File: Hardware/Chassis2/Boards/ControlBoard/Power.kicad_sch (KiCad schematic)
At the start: 4 parts, among them U7 BTS462TATMA1, U8 BTS462TATMA1

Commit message: update hw revision 7
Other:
- company: (none) -> Corzine Lab, University of California, Santa Cruz
- title: (none) -> Open Inverter Platform - Control Board
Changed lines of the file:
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@@
 	(generator "eeschema")
 	(generator_version "10.0")
-	(paper "A4")
+	(paper "USLetter")
+	(title_block
+		(title "Open Inverter Platform - Control Board")
+		(date "2026-07-07")
+		(rev "G")
+		(company "Corzine Lab, University of California, Santa Cruz")
+		(comment 1 "Prepared by Thomas Liao")
+	)
 	(text "3.3V POWER, 3W MAX"
 		(exclude_from_sim no)

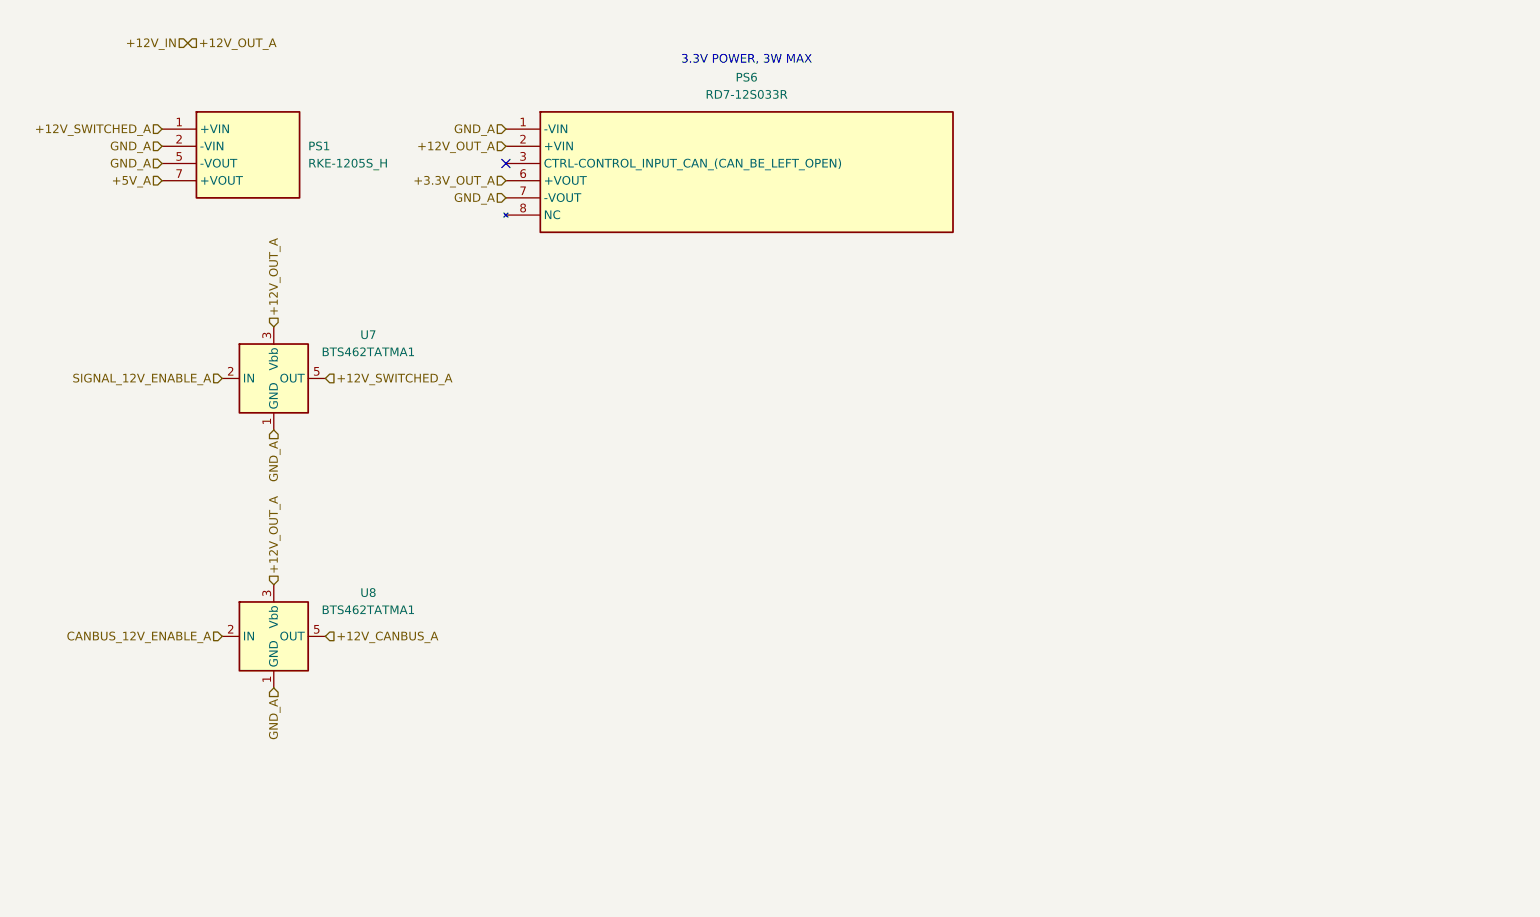
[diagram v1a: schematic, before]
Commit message: eod 2026-07-08
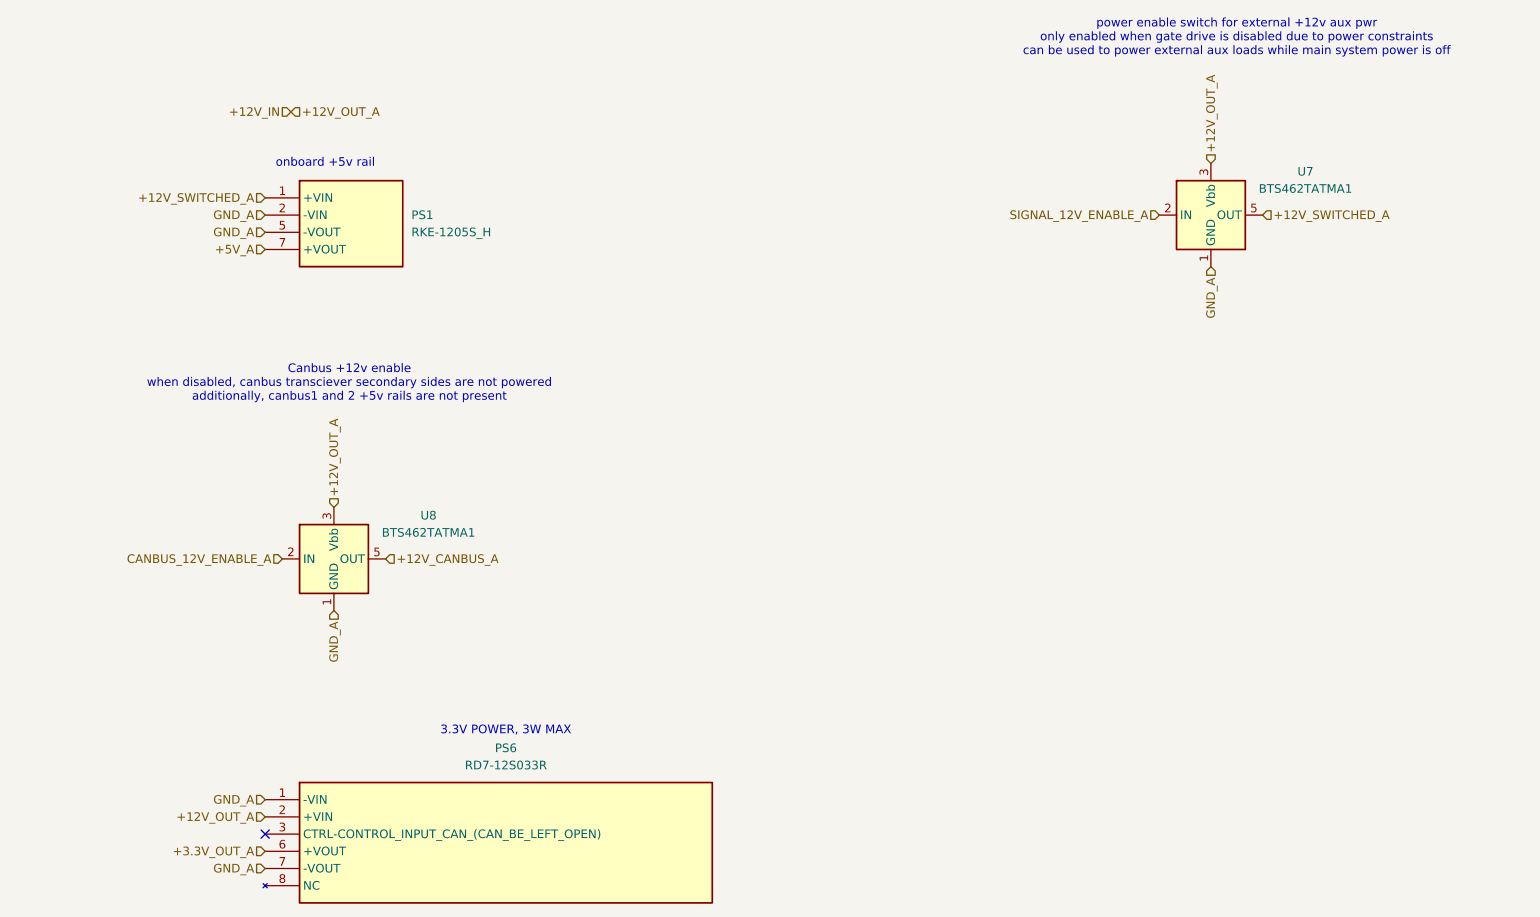
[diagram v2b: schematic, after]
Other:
- note added: "Canbus +12v enable when disabled, canbus transciever secondary sides are not powered additionally, canbus1 and 2 +5v rails are not present"
- note added: "onboard +5v rail"
- note added: "power enable switch for external +12v aux pwr only enabled when gate drive is disabled due to power constraints can be used to power external aux loads while main system power is off"
- moved on the sheet: PS1, PS6, U7, U8
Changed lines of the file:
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@@
 	(text "3.3V POWER, 3W MAX"
 		(exclude_from_sim no)
-		(at 116.84 20.32 0)
+		(at 81.28 119.38 0)
+		(effects
+			(font
+				(size 1.27 1.27)
+			)
+		)
+	)
+	(text "power enable switch for external +12v aux pwr\nonly enabled when gate drive is disabled due to power constraints\ncan be used to power external aux loads while main system power is off"
+		(exclude_from_sim no)
+		(at 189.23 17.018 0)
+		(effects
+			(font
+				(size 1.27 1.27)
+			)
+		)
+	)
+	(text "onboard +5v rail"
+		(exclude_from_sim no)
+		(at 54.61 35.56 0)
+		(effects
+			(font
+				(size 1.27 1.27)
+			)
+		)
+	)
+	(text "Canbus +12v enable\nwhen disabled, canbus transciever secondary sides are not powered\nadditionally, canbus1 and 2 +5v rails are not present"
+		(exclude_from_sim no)
+		(at 58.166 68.072 0)
 		(effects
 			(font
@@
 	)
 	(no_connect
-		(at 81.28 35.56)
+		(at 45.72 134.62)
 	)
 	(hierarchical_label "+12V_OUT_A"
 		(shape input)
-		(at 34.29 17.78 0)
+		(at 49.53 27.94 0)
 		(effects
 			(font
@@
 	(hierarchical_label "CANBUS_12V_ENABLE_A"
 		(shape input)
-		(at 39.37 105.41 180)
+		(at 48.26 93.98 180)
 		(effects
 			(font
@@
 	(hierarchical_label "+12V_SWITCHED_A"
 		(shape input)
-		(at 30.48 30.48 180)
+		(at 45.72 40.64 180)
 		(effects
 			(font
@@
 	(hierarchical_label "+5V_A"
 		(shape input)
-		(at 30.48 38.1 180)
+		(at 45.72 48.26 180)
 		(effects
 			(font
@@
 	(hierarchical_label "GND_A"
 		(shape input)
-		(at 46.99 113.03 270)
+		(at 55.88 101.6 270)
 		(effects
 			(font
@@
 	(hierarchical_label "+12V_OUT_A"
 		(shape input)
-		(at 46.99 59.69 90)
+		(at 185.42 35.56 90)
 		(effects
 			(font
@@
 	(hierarchical_label "GND_A"
 		(shape input)
-		(at 81.28 40.64 180)
+		(at 45.72 139.7 180)
 		(effects
 			(font
@@
 	(hierarchical_label "+12V_CANBUS_A"
 		(shape input)
-		(at 54.61 105.41 0)
+		(at 63.5 93.98 0)
 		(effects
 			(font
@@
 	(hierarchical_label "GND_A"
 		(shape input)
-		(at 30.48 33.02 180)
+		(at 45.72 43.18 180)
 		(effects
 			(font
@@
 	(hierarchical_label "GND_A"
 		(shape input)
-		(at 30.48 35.56 180)
+		(at 45.72 45.72 180)
 		(effects
 			(font
@@
 	(hierarchical_label "+12V_OUT_A"
 		(shape input)
-		(at 46.99 97.79 90)
+		(at 55.88 86.36 90)
 		(effects
 			(font
@@
 	(hierarchical_label "+3.3V_OUT_A"
 		(shape input)
-		(at 81.28 38.1 180)
+		(at 45.72 137.16 180)
 		(effects
 			(font
@@
 	(hierarchical_label "GND_A"
 		(shape input)
-		(at 46.99 74.93 270)
+		(at 185.42 50.8 270)
 		(effects
 			(font
@@
 	(hierarchical_label "+12V_SWITCHED_A"
 		(shape input)
-		(at 54.61 67.31 0)
+		(at 193.04 43.18 0)
 		(effects
 			(font
@@
 	(hierarchical_label "GND_A"
 		(shape input)
-		(at 81.28 30.48 180)
+		(at 45.72 129.54 180)
 		(effects
 			(font
@@
 	(hierarchical_label "+12V_IN"
 		(shape input)
-		(at 34.29 17.78 180)
+		(at 49.53 27.94 180)
 		(effects
 			(font
@@
 	(hierarchical_label "+12V_OUT_A"
 		(shape input)
-		(at 81.28 33.02 180)
+		(at 45.72 132.08 180)
 		(effects
 			(font
@@
 	(hierarchical_label "SIGNAL_12V_ENABLE_A"
 		(shape input)
-		(at 39.37 67.31 180)
+		(at 177.8 43.18 180)
 		(effects
 			(font
@@
 	(symbol
 		(lib_id "Power_Management:BTS462TATMA1")
-		(at 46.99 67.31 0)
+		(at 185.42 43.18 0)
 		(unit 1)
 		(body_style 1)
@@
 		(fields_autoplaced yes)
 		(property "Reference" "U7"
-			(at 60.96 60.8898 0)
+			(at 199.39 36.7598 0)
 			(show_name no)
 			(do_not_autoplace no)
@@
 		)
 		(property "Value" "BTS462TATMA1"
-			(at 60.96 63.4298 0)
+			(at 199.39 39.2998 0)
 			(show_name no)
 			(do_not_autoplace no)
@@
 		)
 		(property "Footprint" "Package_TO_SOT_SMD:TO-252-4"
-			(at 46.99 87.63 0)
+			(at 185.42 63.5 0)
 			(hide yes)
 			(show_name no)
@@
 		)
 		(property "Datasheet" "https://www.infineon.com/dgdl/Infineon-BTS462T-DS-v01_01-EN.pdf?fileId=5546d4625a888733015aa9b0294035f6"
-			(at 46.99 90.17 0)
+			(at 185.42 66.04 0)
 			(hide yes)
 			(show_name no)
@@
 		)
 		(property "Description" "Smart High-Side Power Switch, PROFET, Single, 100mOhm, 3.5A, 34V, TO-252-4"
-			(at 46.99 67.31 0)
+			(at 185.42 43.18 0)
 			(hide yes)
 			(show_name no)
@@
 	(symbol
 		(lib_id "Power_Management:BTS462TATMA1")
-		(at 46.99 105.41 0)
+		(at 55.88 93.98 0)
 		(unit 1)
 		(body_style 1)
@@
 		(fields_autoplaced yes)
 		(property "Reference" "U8"
-			(at 60.96 98.9898 0)
+			(at 69.85 87.5598 0)
 			(show_name no)
 			(do_not_autoplace no)
@@
 		)
 		(property "Value" "BTS462TATMA1"
-			(at 60.96 101.5298 0)
+			(at 69.85 90.0998 0)
 			(show_name no)
 			(do_not_autoplace no)
@@
 		)
 		(property "Footprint" "Package_TO_SOT_SMD:TO-252-4"
-			(at 46.99 125.73 0)
+			(at 55.88 114.3 0)
 			(hide yes)
 			(show_name no)
@@
 		)
 		(property "Datasheet" "https://www.infineon.com/dgdl/Infineon-BTS462T-DS-v01_01-EN.pdf?fileId=5546d4625a888733015aa9b0294035f6"
-			(at 46.99 128.27 0)
+			(at 55.88 116.84 0)
 			(hide yes)
 			(show_name no)
@@
 		)
 		(property "Description" "Smart High-Side Power Switch, PROFET, Single, 100mOhm, 3.5A, 34V, TO-252-4"
-			(at 46.99 105.41 0)
+			(at 55.88 93.98 0)
 			(hide yes)
 			(show_name no)
@@
 	(symbol
 		(lib_id "InverterCom:RKE-1205S_H")
-		(at 30.48 30.48 0)
+		(at 45.72 40.64 0)
 		(unit 1)
 		(body_style 1)
@@
 		(fields_autoplaced yes)
 		(property "Reference" "PS1"
-			(at 52.07 33.0199 0)
+			(at 67.31 43.1799 0)
 			(show_name no)
 			(do_not_autoplace no)
@@
 		)
 		(property "Value" "RKE-1205S_H"
-			(at 52.07 35.5599 0)
+			(at 67.31 45.7199 0)
 			(show_name no)
 			(do_not_autoplace no)
@@
 		)
 		(property "Footprint" "InverterCom:RKE1205SH"
-			(at 52.07 125.4 0)
+			(at 67.31 135.56 0)
 			(hide yes)
 			(show_name no)
@@
 		)
 		(property "Datasheet" "https://www.recom-power.com/pdf/Econoline/RKE.pdf"
-			(at 52.07 225.4 0)
+			(at 67.31 235.56 0)
 			(hide yes)
 			(show_name no)
@@
 		)
 		(property "Description" "Recom Through Hole 1W Isolated DC-DC Converter, Vin Maximum of 12 V dc, I/O isolation 4kV dc, Vout 5V dc"
-			(at 30.48 30.48 0)
+			(at 45.72 40.64 0)
 			(hide yes)
 			(show_name no)
@@
 		)
 		(property "Height" "10.7"
-			(at 52.07 425.4 0)
+			(at 67.31 435.56 0)
 			(hide yes)
 			(show_name no)
@@
 		)
 		(property "Mouser Part Number" "919-RKE-1205S/H"
-			(at 52.07 525.4 0)
+			(at 67.31 535.56 0)
 			(hide yes)
 			(show_name no)
@@
 		)
 		(property "Mouser Price/Stock" "https://www.mouser.co.uk/ProductDetail/RECOM-Power/RKE-1205S-H?qs=IFMNCcK%2FBZwj8OgeraTUUA%3D%3D"
-			(at 52.07 625.4 0)
+			(at 67.31 635.56 0)
 			(hide yes)
 			(show_name no)
@@
 		)
 		(property "Manufacturer_Name" "RECOM Power"
-			(at 52.07 725.4 0)
+			(at 67.31 735.56 0)
 			(hide yes)
 			(show_name no)
@@
 		)
 		(property "Manufacturer_Part_Number" "RKE-1205S/H"
-			(at 52.07 825.4 0)
+			(at 67.31 835.56 0)
 			(hide yes)
 			(show_name no)
@@
 	(symbol
 		(lib_id "InverterCom:RD7-12S033R")
-		(at 81.28 30.48 0)
+		(at 45.72 129.54 0)
 		(unit 1)
 		(body_style 1)
@@
 		(fields_autoplaced yes)
 		(property "Reference" "PS6"
-			(at 116.84 22.86 0)
+			(at 81.28 121.92 0)
 			(show_name no)
 			(do_not_autoplace no)
@@
 		)
 		(property "Value" "RD7-12S033R"
-			(at 116.84 25.4 0)
+			(at 81.28 124.46 0)
 			(show_name no)
 			(do_not_autoplace no)
@@
 		)
 		(property "Footprint" "InverterCom:RD712S033R"
-			(at 148.59 125.4 0)
+			(at 113.03 224.46 0)
 			(hide yes)
 			(show_name no)
@@
 		)
 		(property "Datasheet" "https://app.adam-tech.com/products/download/data_sheet/247025/rd7-12s033r-data-sheet.pdf"
-			(at 148.59 225.4 0)
+			(at 113.03 324.46 0)
 			(hide yes)
 			(show_name no)
@@
 		)
 		(property "Description" "Isolated DC/DC Converters - Through Hole DC-DC Converter, Isolated Module, Single Output, 9V-18VDC Input, 3.3VDC, 3W"
-			(at 81.28 30.48 0)
+			(at 45.72 129.54 0)
 			(hide yes)
 			(show_name no)
@@
 		)
 		(property "Height" "11.6"
-			(at 148.59 425.4 0)
+			(at 113.03 524.46 0)
 			(hide yes)
 			(show_name no)
@@
 		)
 		(property "Mouser Part Number" ""
-			(at 148.59 525.4 0)
+			(at 113.03 624.46 0)
 			(hide yes)
 			(show_name no)
@@
 		)
 		(property "Mouser Price/Stock" ""
-			(at 148.59 625.4 0)
+			(at 113.03 724.46 0)
 			(hide yes)
 			(show_name no)
@@
 		)
 		(property "Manufacturer_Name" "Adam Tech"
-			(at 148.59 725.4 0)
+			(at 113.03 824.46 0)
 			(hide yes)
 			(show_name no)
@@
 		)
 		(property "Manufacturer_Part_Number" "RD7-12S033R"
-			(at 148.59 825.4 0)
-			(hide yes)
-			(show_name no)
+			(at 113.03 924.46 0)
+			(hide yes)
+			(show_name no)

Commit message: Labels tool, composite board views, InverterGen5 C2 branding, even render resolution
- Labels.pdf: HV warning labels, chassis ID, per-assembly labels (label cmd)
- Board sections add composite front/back views (PCB-viewer look, mirrored
  back) and layer plots now carry the drawing sheet with true plot scale
- Branding standardized to InverterGen5 C2 (cover, footer, labels)
- STEP previews render at even resolution regardless of part aspect
- Fab part titles from info.txt PartName; ALL-CAPS handling fixed
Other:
- title: Open Inverter Platform - Control Board -> InverterGen5 - Control Board
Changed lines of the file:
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@@
 	(paper "USLetter")
 	(title_block
-		(title "Open Inverter Platform - Control Board")
+		(title "InverterGen5 - Control Board")
 		(date "2026-07-07")
 		(rev "A")

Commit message: Vendor BTS462TATMA1 symbol into InverterCom library
The symbol was referenced as Power_Management:BTS462TATMA1, which is
not vendored (project sym-lib-table only registers InverterCom) so
resolution silently depended on the machine's global KiCad symbol
libs. Copied the BTS462TATMA1 symbol verbatim from the installed
KiCad 10.0.3 stock library (self-contained, no extends; footprint
property stays Package_TO_SOT_SMD:TO-252-4, a stock global footprint)
into PartsLib/InverterCom.kicad_sym and repointed all lib_ids and
embedded lib_symbols copies (Chassis2 Power.kicad_sch, PowerSwitch
.kicad_sch, IOBoard.kicad_sch; SECC CableIO.kicad_sch) to
InverterCom:BTS462TATMA1. Vendored copy is byte-identical in content
to the embedded cached copies.
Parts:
- U7, U8: symbol Power_Management:BTS462TATMA1 -> InverterCom:BTS462TATMA1
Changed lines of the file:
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@@
 	)
 	(symbol
-		(lib_id "Power_Management:BTS462TATMA1")
+		(lib_id "InverterCom:BTS462TATMA1")
 		(at 185.42 43.18 0)
 		(unit 1)
@@
 	)
 	(symbol
-		(lib_id "Power_Management:BTS462TATMA1")
+		(lib_id "InverterCom:BTS462TATMA1")
 		(at 55.88 93.98 0)
 		(unit 1)
